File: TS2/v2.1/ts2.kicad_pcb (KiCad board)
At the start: 2 copper layers, 134.6 x 208.3 mm, 110 parts, among them P1 FTDI (TERMINAL), P2 FTDI (HOST), P3 +5V POWER, SW1 RESET, SW2 SINGLE STEP/RUN, SW3 STEP, SW4 ABORT, SW5 POWER, U1 555, U10 74LS32, U11 HM6264, U12 28C64, U13 HM6264, U14 28C64, U15 HM6264, U16 28C64, U17 HM6264, U18 28C64, U19 74LS20, U2 8 MHz, U20 74LS74, U21 74LS161, U22 74LS161, U23 74LS74, U24 74LS260, U25 74LS260, U26 74LS138, U27 74LS138, U28 74LS148, U29 6850, U3 74LS00, U30 6850, U31 74HC4060, U32 74LS138, U33 74LS138, U34 74LS00, U35 74LS74, U36 74LS27, U37 74LS00, U4 74LS06, U5 74LS04, U6 68000, U7 74LS08, U8 74LS32, U9 74LS32, Y1 2.4576MHz

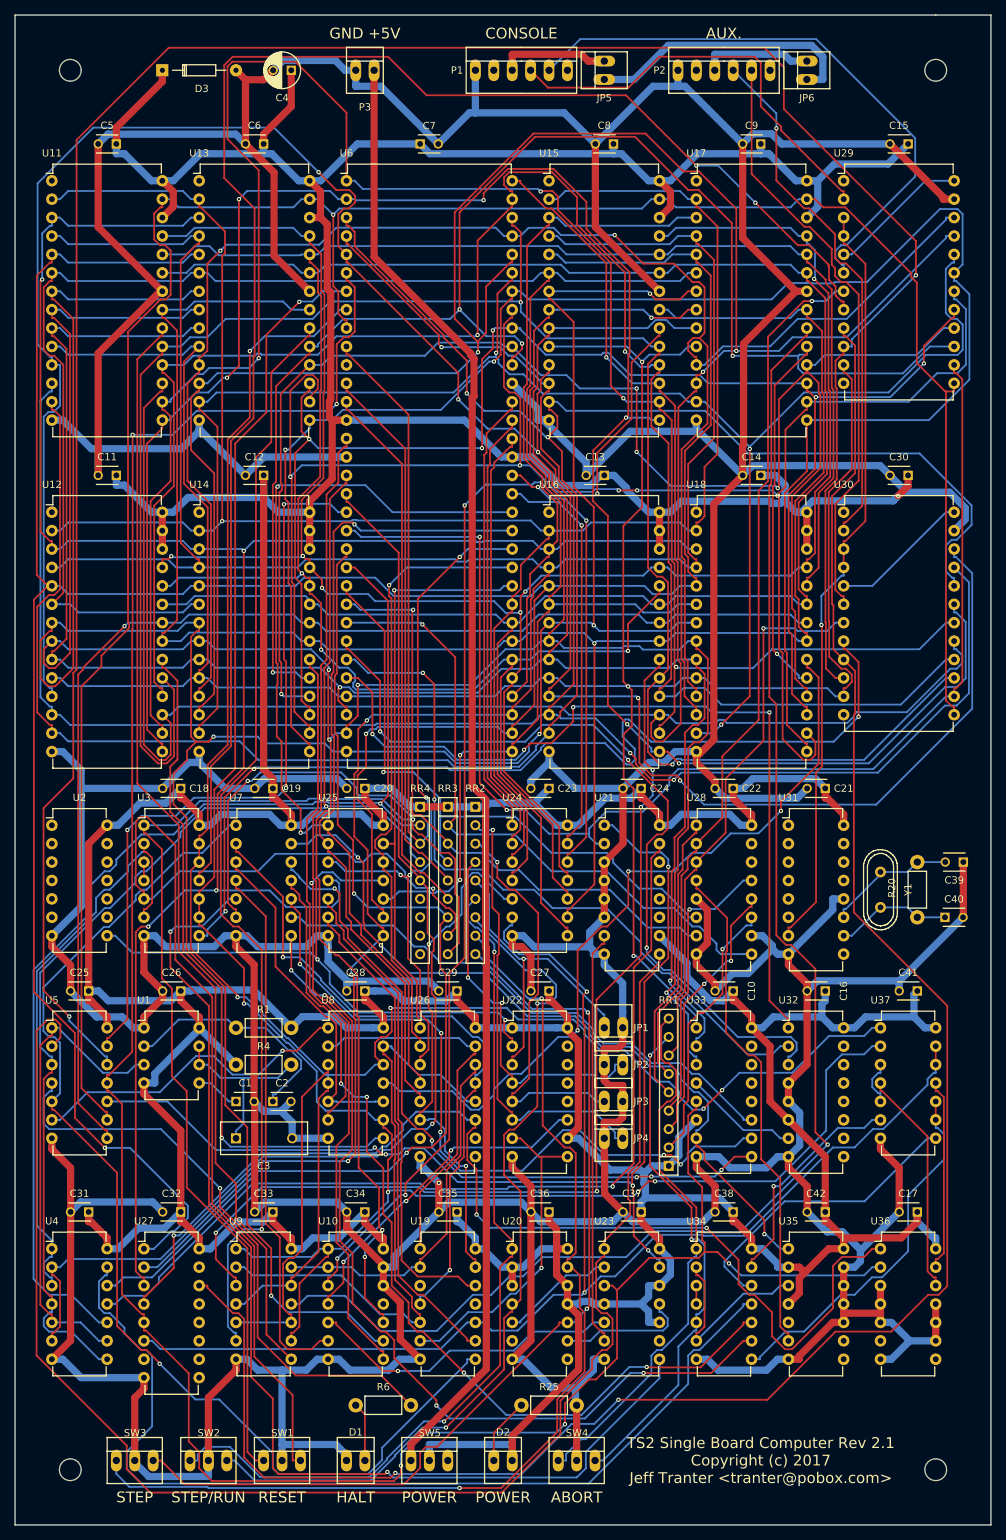
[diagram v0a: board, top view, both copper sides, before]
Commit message: Rev 2.1.1 changes.
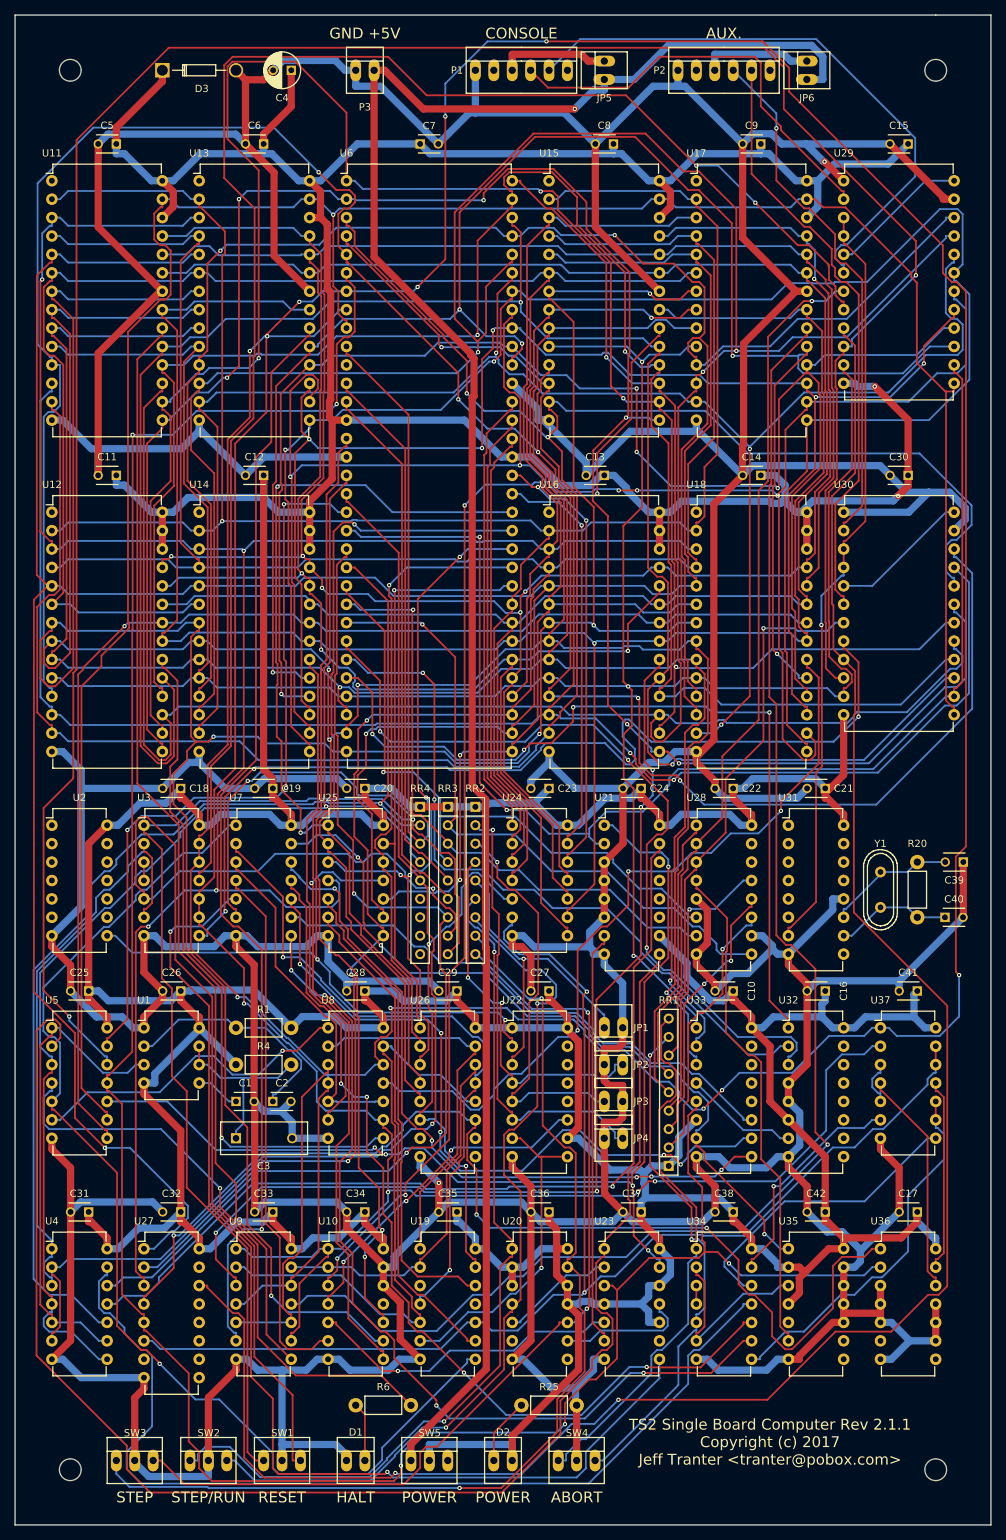
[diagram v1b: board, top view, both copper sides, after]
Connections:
- P3 pad 2: Net-(P3-Pad2) -> POWER
- SW5 pad 1: Net-(P3-Pad2) -> POWER
- U29 pad 1: (no net) -> GND
- U29 pad 12: (no net) -> VCC
- U30 pad 1: (no net) -> GND
- U30 pad 12: (no net) -> VCC
- U6 pad 7: LDS* -> UDS*
- U6 pad 8: UDS* -> LDS*
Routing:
- net UDS*: track 265.0 -> 561.0 mm, vias 5 -> 9
- net POWER: track 38.1 -> 277.3 mm, vias 0 -> 1
- net Net-(P3-Pad2): track 202.7 -> 0.00 mm
- net LDS*: track 274.4 -> 224.2 mm, vias 5 -> 6
- net VCC: track 1108.4 -> 1139.0 mm, vias 1 -> 2
- net GND: track 1388.1 -> 1408.3 mm, vias 1 -> 2
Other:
- board text added: "TS2 Single Board Computer Rev 2.1.1 Copyright (c) 2017 Jeff Tranter <tranter@pobox.com>"
- board text removed: "TS2 Single Board Computer Rev 2.1 Copyright (c) 2017 Jeff Tranter <tranter@pobox.com>"
